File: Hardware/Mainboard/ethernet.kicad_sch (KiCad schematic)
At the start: 2 parts, among them J12 ARJM11D7-009-AB-EW2, U1 ENC624J600-I/PT

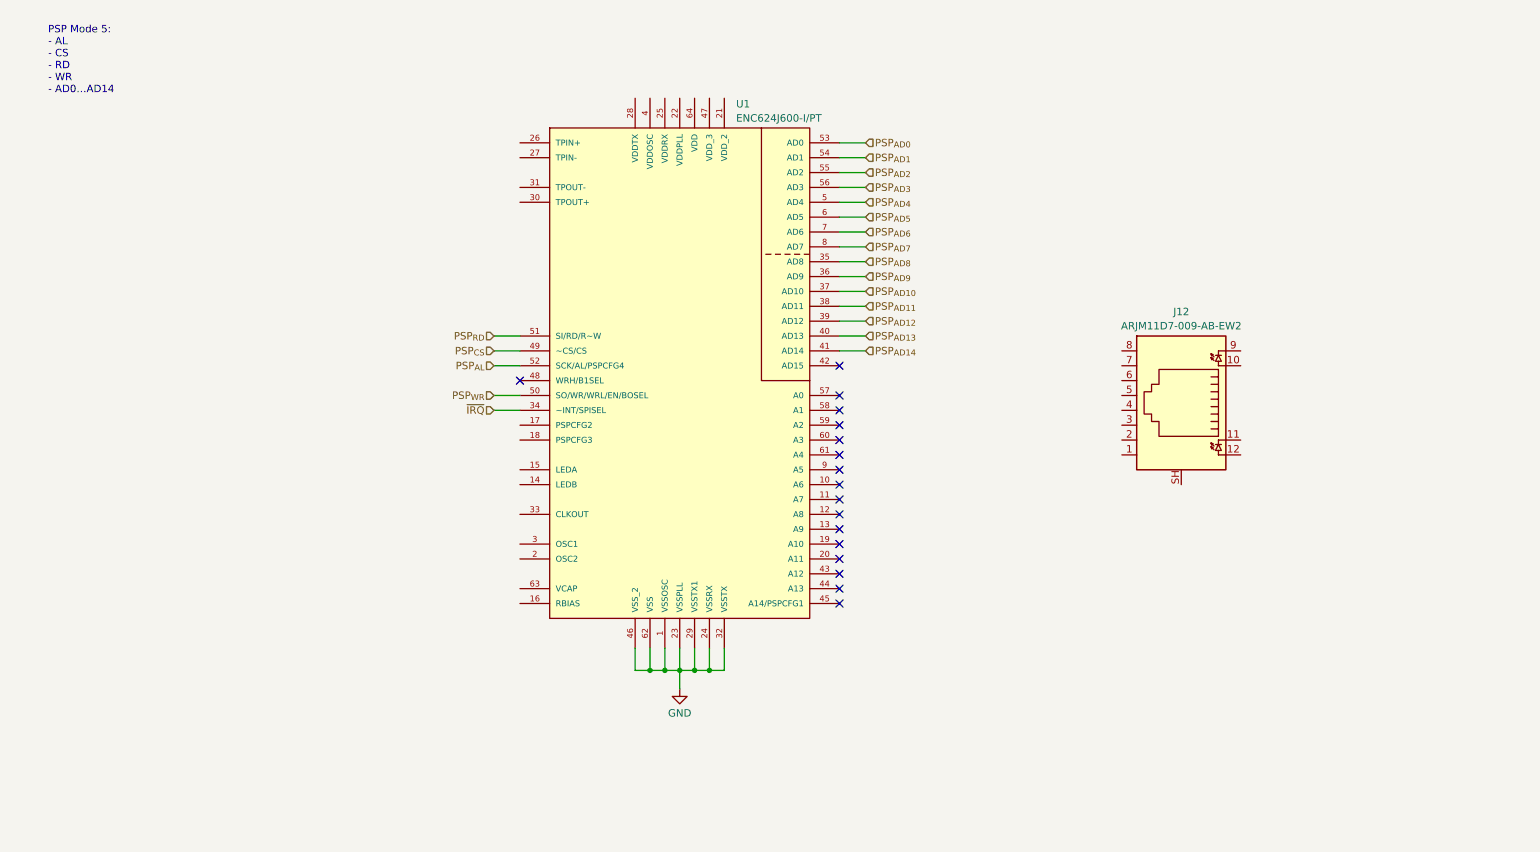
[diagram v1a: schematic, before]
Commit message: More work on the motherboard
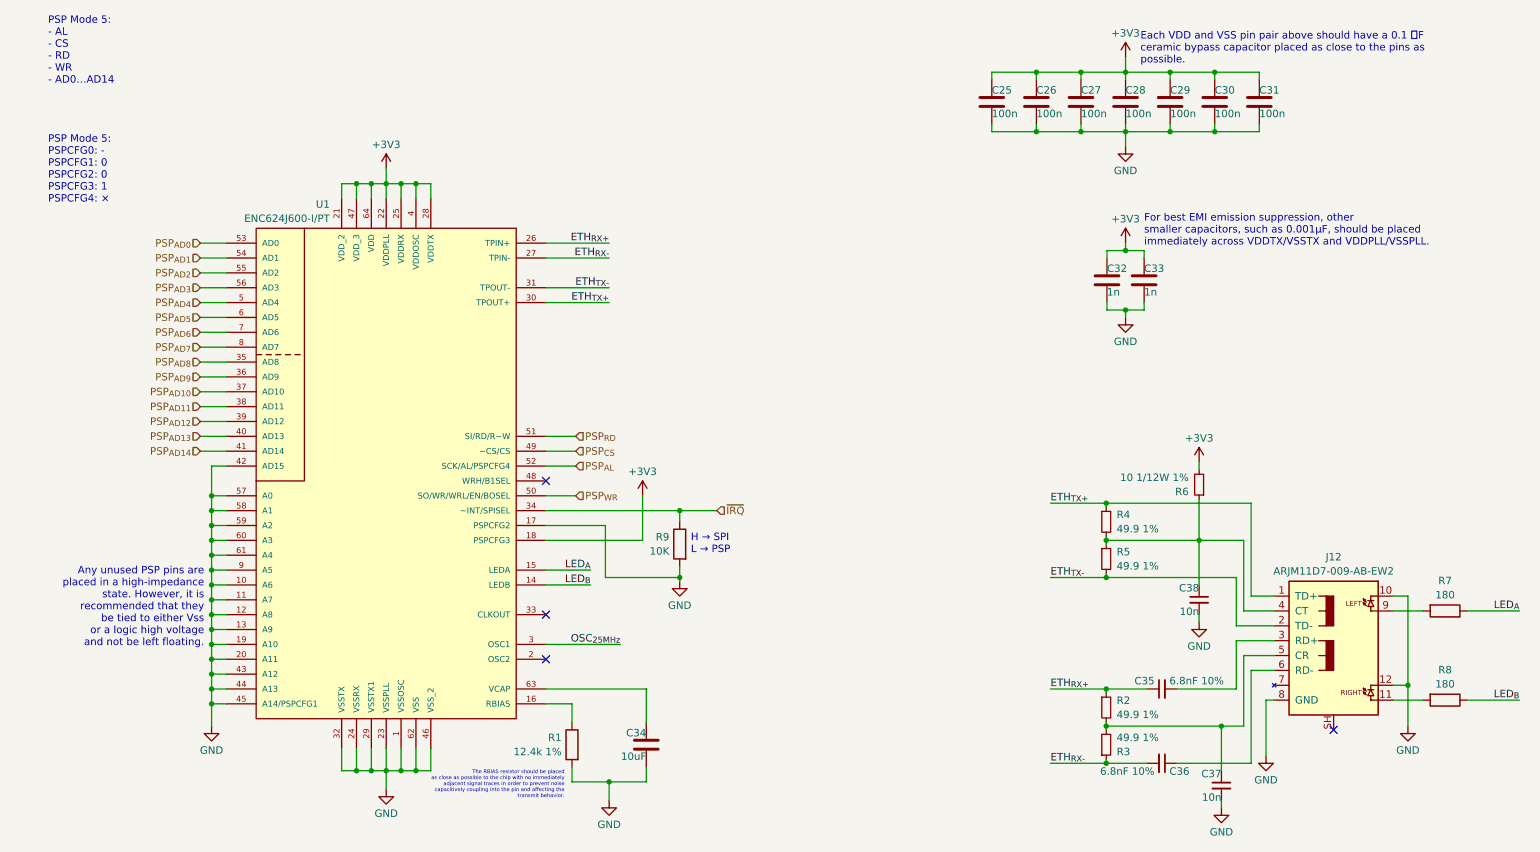
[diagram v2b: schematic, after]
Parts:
- added C25, C26, C27, C28, C29, C30, C31: 100n, Capacitor_SMD:C_0603_1608Metric_Pad1.08x0.95mm_HandSolder, symbol Device:C
- added C32, C33: 1n, Capacitor_SMD:C_0603_1608Metric_Pad1.08x0.95mm_HandSolder, symbol Device:C
- added C34: 10uF, Capacitor_SMD:C_0603_1608Metric_Pad1.08x0.95mm_HandSolder, symbol Device:C
- added C35, C36: 6.8nF 10%, Capacitor_SMD:C_0603_1608Metric_Pad1.08x0.95mm_HandSolder, symbol Device:C_Small
- added C37, C38: 10n, Capacitor_SMD:C_0603_1608Metric_Pad1.08x0.95mm_HandSolder, symbol Device:C_Small
- added R1: 12.4k 1%, symbol Device:R
- added R2, R3, R4, R5: 49.9 1%, Resistor_SMD:R_0603_1608Metric_Pad0.98x0.95mm_HandSolder, symbol Device:R_Small
- added R6: 10 1/12W 1%, Resistor_SMD:R_0603_1608Metric_Pad0.98x0.95mm_HandSolder, symbol Device:R_Small
- added R7, R8: 180, symbol Device:R
- added R9: 10K, symbol Device:R
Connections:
- net GND: now also J12.10, J12.12, J12.8 (GND), U1.10 (A6), U1.11 (A7), U1.12 (A8), U1.13 (A9), U1.17 (PSPCFG2), U1.19 (A10), U1.20 (A11), U1.42 (AD15), U1.43 (A12), U1.44 (A13), U1.45 (A14/PSPCFG1), U1.57 (A0), U1.58 (A1), U1.59 (A2), U1.60 (A3), U1.61 (A4), U1.9 (A5), C25.2, C26.2, C27.2, C28.2, C29.2, C30.2, C31.2, C32.2, C33.2, C34.2, C37.2, C38.2, R1.2, R9.2
- net ~{IRQ}: now also R9.1
- net ETH_{TX+}: now reaches J12.1 (TD+)
- net ETH_{TX+}: now also U1.30 (TPOUT+), R4.1
- net at J12.11: now also R8.2
- net ETH_{TX-}: now reaches J12.2 (TD-)
- net ETH_{TX-}: now also U1.31 (TPOUT-), R5.2
- net at J12.3 (RD+): now also C35.2
- net at J12.4 (CT): now also C38.1, R4.2, R5.1, R6.1
- net at J12.5 (CR): now also C37.1, R2.2, R3.2
- net at J12.6 (RD-): now also C36.1
- net at J12.9: now also R7.2
- net LED_{B}: now reaches U1.14 (LEDB)
- net LED_{B}: now also R8.1
- net LED_{A}: now reaches U1.15 (LEDA)
- net LED_{A}: now also R7.1
- net at U1.16 (RBIAS): now also R1.1
- net +3V3: now reaches U1.18 (PSPCFG3)
- net +3V3: now also U1.21 (VDD_2), U1.22 (VDDPLL), U1.25 (VDDRX), U1.28 (VDDTX), U1.4 (VDDOSC), U1.47 (VDD_3), U1.64 (VDD), C25.1, C26.1, C27.1, C28.1, C29.1, C30.1, C31.1, C32.1, C33.1, R6.2
- net ETH_{RX+}: now reaches U1.26 (TPIN+)
- net ETH_{RX+}: now also C35.1, R2.1
- net ETH_{RX-}: now reaches U1.27 (TPIN-)
- net ETH_{RX-}: now also C36.2, R3.1
- net OSC_{25MHz}: now reaches U1.3 (OSC1)
- net at U1.63 (VCAP): now also C34.1
- no-connect marks 17 -> 4
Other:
- note added: "Any unused PSP pins are placed in a high-impedance state. However, it is recommended that they be tied to either Vss or a logic high voltage and not be left floating."
- note added: "Each VDD and VSS pin pair above should have a 0.1 F ceramic bypass capacitor placed as close to the pins as possible."
- note added: "For best EMI emission suppression, other smaller capacitors, such as 0.001µF, should be placed immediately across VDDTX/VSSTX and VDDPLL/VSSPLL."
- note added: "H → SPI L → PSP"
- note added: "PSP Mode 5: PSPCFG0: - PSPCFG1: 0 PSPCFG2: 0 PSPCFG3: 1 PSPCFG4: ×"
- note added: "The RBIAS resistor should be placed as close as possible to the chip with no immediately adjacent signal traces in order to prevent noise capacitively coupling into the pin and affecting the transmit behavior."
- moved on the sheet: U1
